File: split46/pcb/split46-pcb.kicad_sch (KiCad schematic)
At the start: 55 parts, among them J1 AudioJack4, SW1 SW_SPST, SW10 SW_SPST, SW11 SW_SPST, SW12 SW_SPST, SW13 SW_SPST, SW14 SW_SPST, SW15 SW_SPST, SW16 SW_SPST, SW17 SW_SPST, SW18 SW_SPST, SW19 SW_SPST, SW2 SW_SPST, SW20 SW_SPST, SW21 SW_SPST, SW22 SW_SPST, SW23 SW_SPST, SW3 SW_SPST, SW4 SW_SPST, SW5 SW_SPST, SW6 SW_SPST, SW7 SW_SPST, SW8 SW_SPST, SW9 SW_SPST, U1 rp2040-zero

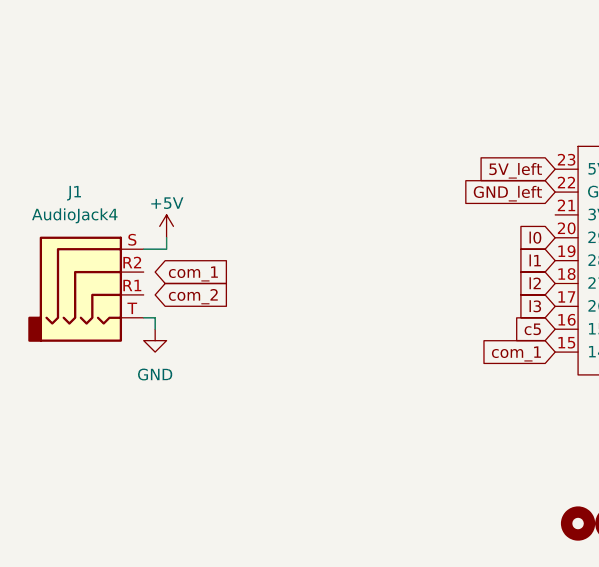
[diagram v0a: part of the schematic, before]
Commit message: dim. 17 mars 2024 09:56:18 CET
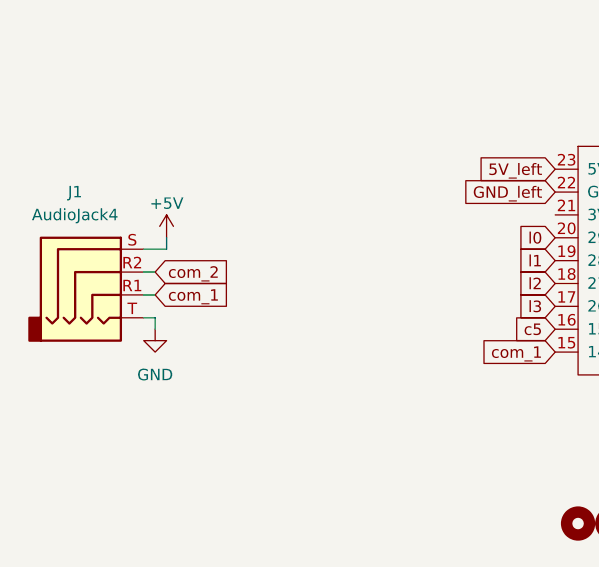
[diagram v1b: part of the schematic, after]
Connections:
- net com_1: now also J1.R1
- net com_2: now also J1.R2
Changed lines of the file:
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@@
+    (stroke (width 0) (type default))
+  )
+  (wire (pts (xy 81.28 82.55) (xy 82.55 82.55))
+    (stroke (width 0) (type default))
+  )
+  (wire (pts (xy 81.28 85.09) (xy 82.55 85.09))
     (stroke (width 0) (type default))
   )
@@
     )
   )
-  (global_label "com_1" (shape input) (at 82.55 82.55 0) (fields_autoplaced)
-    (effects (font (size 1.27 1.27)) (justify left))
-    (property "Intersheetrefs" "${INTERSHEET_REFS}" (at 91.6432 82.55 0)
+  (global_label "com_1" (shape input) (at 82.55 85.09 0) (fields_autoplaced)
+    (effects (font (size 1.27 1.27)) (justify left))
+    (property "Intersheetrefs" "${INTERSHEET_REFS}" (at 91.6432 85.09 0)
       (effects (font (size 1.27 1.27)) (justify left) hide)
     )
@@
     )
   )
-  (global_label "com_2" (shape input) (at 82.55 85.09 0) (fields_autoplaced)
-    (effects (font (size 1.27 1.27)) (justify left))
-    (property "Intersheetrefs" "${INTERSHEET_REFS}" (at 91.5638 85.09 0)
-      (effects (font (size 1.27 1.27)) (justify left) hide)
-    )
+  (global_label "com_2" (shape input) (at 82.55 82.55 0) (fields_autoplaced)
+    (effects (font (size 1.27 1.27)) (justify left))
+    (property "Intersheetrefs" "${INTERSHEET_REFS}" (at 91.5638 82.55 0)
+      (effects (font (size 1.27 1.27)) (justify left) hide)
+    )

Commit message: ""
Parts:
- U1: footprint mcu:rp2040-zero-tht -> _mcu:rp2040-zero-tht
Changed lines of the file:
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@@
       (effects (font (size 1.27 1.27)))
     )
-    (property "Footprint" "mcu:rp2040-zero-tht" (at 130.81 74.93 0)
+    (property "Footprint" "_mcu:rp2040-zero-tht" (at 130.81 74.93 0)
       (effects (font (size 1.27 1.27)) hide)
     )
